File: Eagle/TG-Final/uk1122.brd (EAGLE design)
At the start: 172.7 x 76.2 mm, 2 parts

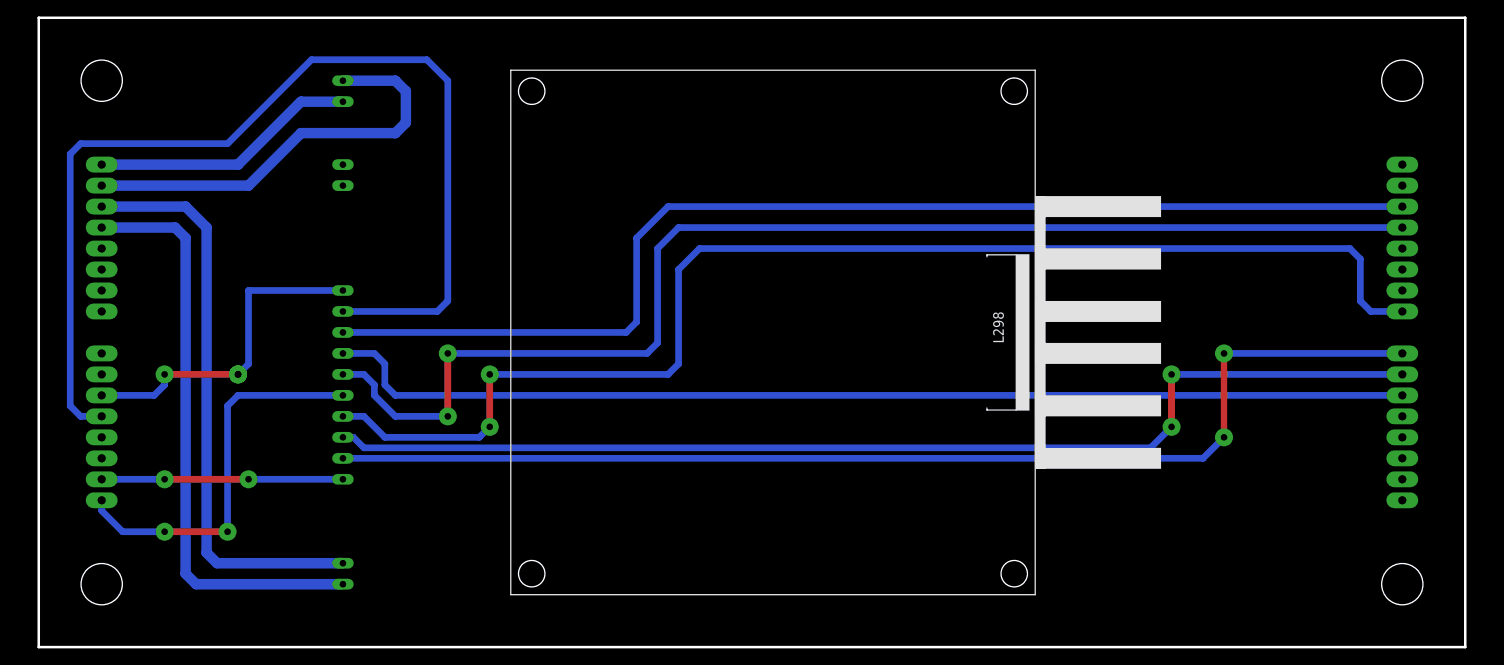
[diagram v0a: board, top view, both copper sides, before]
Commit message: Muchos Cambios a 2 dias de la denfesa
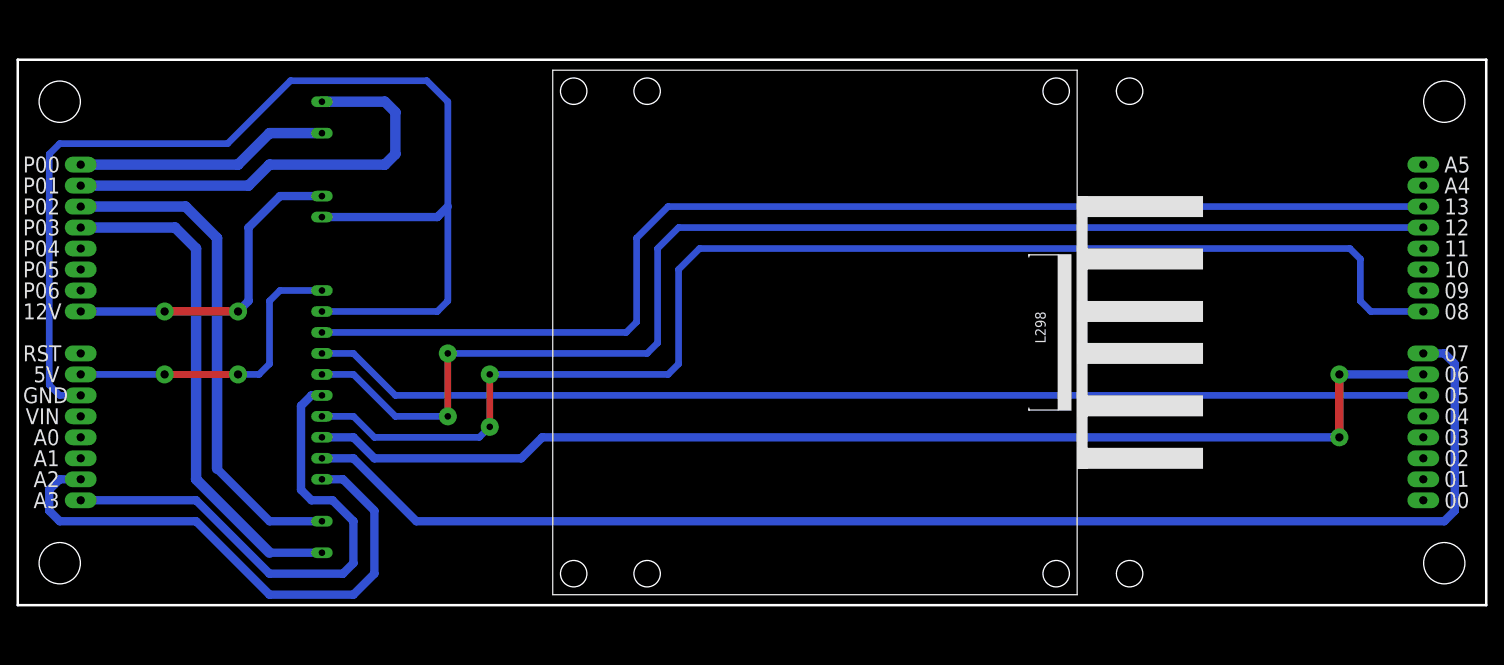
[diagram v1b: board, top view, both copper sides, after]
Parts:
- U$1: value BASEFINAL -> BASE-FINAL
- moved U$2 2.54 mm to (83.8, 36.8)
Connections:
- removed net +: U$2.+
- removed net -: U$2.-
- removed net N$12: U$1.P$24, U$2.IN4
- removed net N$14: U$1.P$15, U$2.CSB
- removed net N$3: U$1.P$3, U$2.MOT2R
- removed net N$4: U$1.P$4, U$2.MOT2A
- new net CSB: U$1.A2, U$2.CSB
- new net IN4: U$1.7, U$2.IN4
- new net MOT2A: U$1.PIN03, U$2.MOT2A
- new net MOT2R: U$1.PIN02, U$2.MOT2R
- new net N$21: U$1.GND, U$2.+5, U$2.-
- net N$1: now also U$1.PIN00; no longer U$1.P$1
- net N$10: now also U$1.A3; no longer U$1.P$16
- net N$11: now also U$1.8; no longer U$1.P$25
- net N$13: now also U$1.6; no longer U$1.P$23
- net N$2: now also U$1.PIN01; no longer U$1.P$2
- net N$5: now also U$1.5V; no longer U$1.P$11
- net N$6: now also U$1.12V, U$2.+; no longer U$1.P$12, U$2.+5
- net N$7: now also U$1.13; no longer U$1.P$30
- net N$8: now also U$1.12; no longer U$1.P$29
- net N$9: now also U$1.5; no longer U$1.P$22
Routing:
- net IN4: track 0.00 -> 163.0 mm
- net N$21: track 0.00 -> 140.9 mm
- net N$12: track 139.5 -> 0.00 mm, vias 1 -> 0
- net N$6: track 126.2 -> 40.2 mm, vias 0 -> 2
- net N$4: track 70.9 -> 0.00 mm
- net N$3: track 70.2 -> 0.00 mm
- net CSB: track 0.00 -> 67.1 mm
- net MOT2A: track 0.00 -> 61.9 mm
- net MOT2R: track 0.00 -> 61.4 mm
- net N$14: track 29.2 -> 0.00 mm
- net N$10: track 47.3 -> 63.5 mm, vias 2 -> 0
- net N$13: track 136.2 -> 143.1 mm, vias 1 -> 2
- net N$7: track 140.5 -> 145.6 mm
- net N$11: track 155.3 -> 160.4 mm
- net N$8: track 151.7 -> 156.1 mm
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- added copper zone on layer 16, net N$4
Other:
- board size 172.7 x 76.2 mm -> 177.8 x 66 mm
